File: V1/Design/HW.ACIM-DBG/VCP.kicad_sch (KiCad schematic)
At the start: 18 parts, among them J2 VCP ICSP, U3 PIC32MM0064GPM028

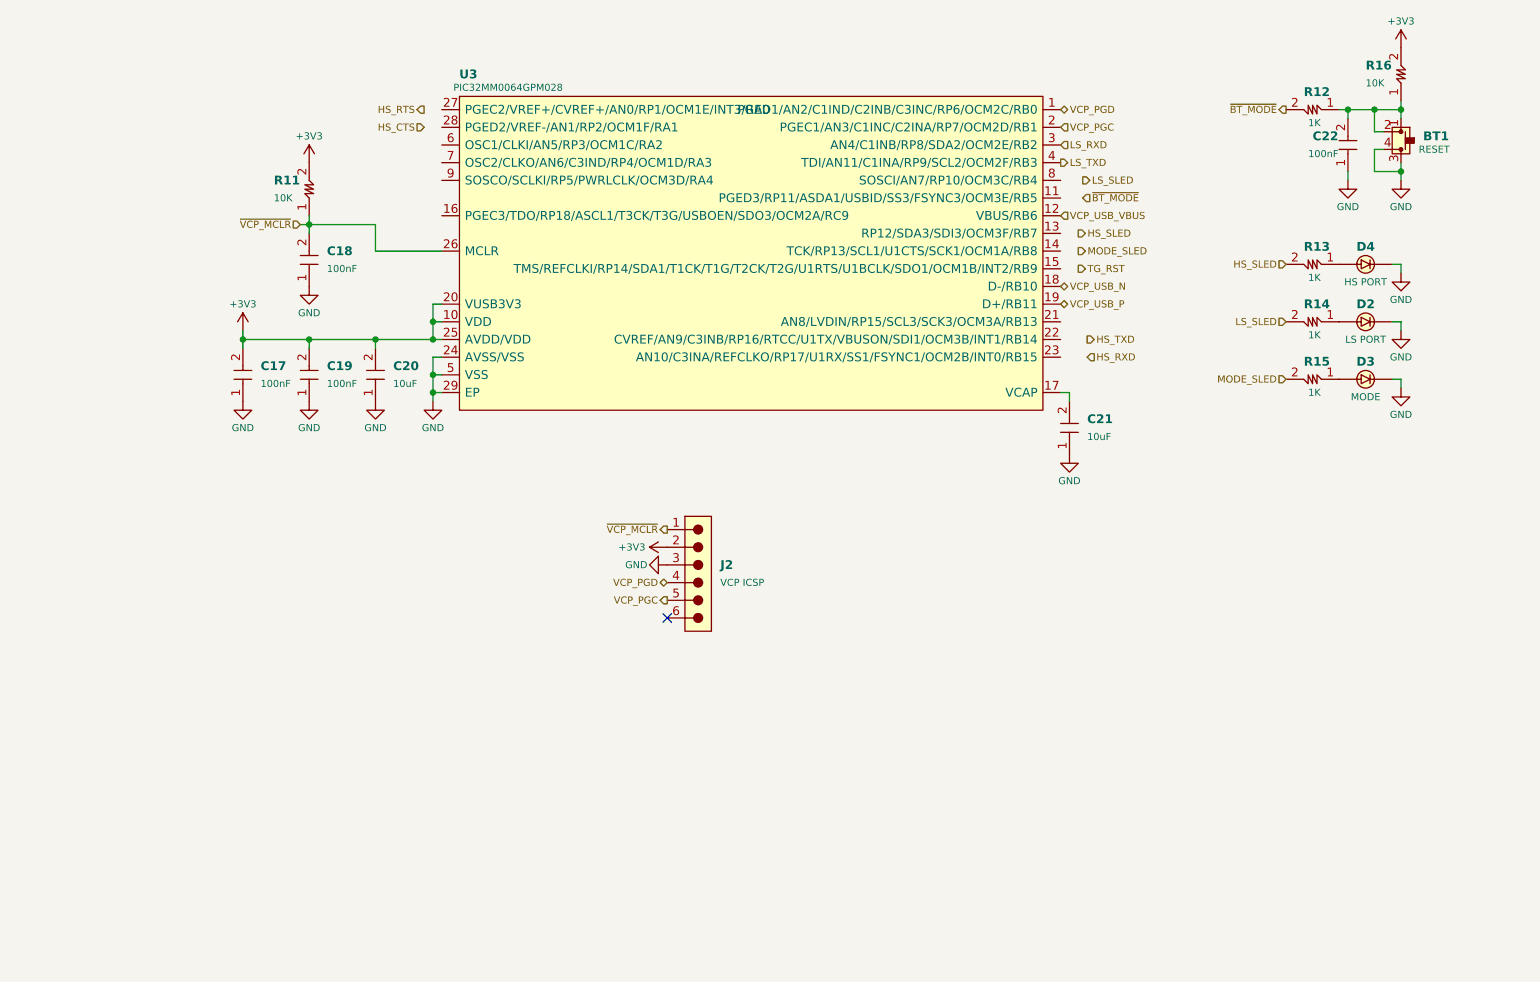
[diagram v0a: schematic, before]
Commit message: V1 layout update 2
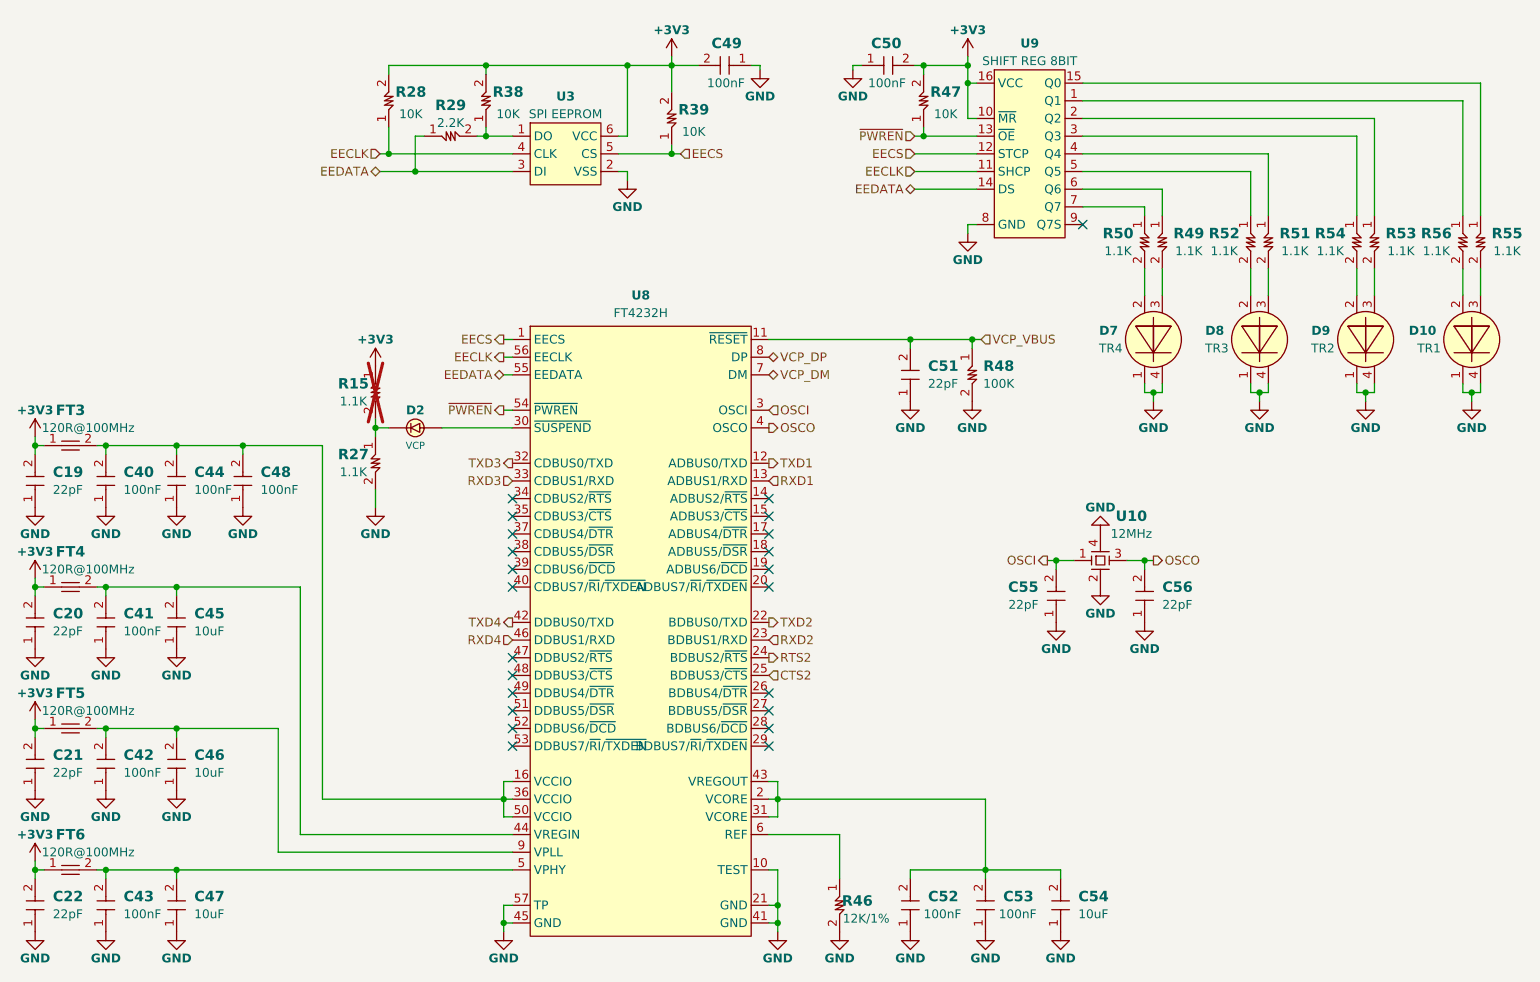
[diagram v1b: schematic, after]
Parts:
- removed BT1: RESET, SAMPI:BUTTON_4P_6x6, symbol SAMPI:BT
- removed C17, C18: 100nF, SAMPI:CAP0603, symbol SAMPI:CERCAP
- removed D3: MODE, SAMPI:LED3MM, symbol SAMPI:RLED
- removed D4: HS PORT, SAMPI:LED3MM, symbol SAMPI:YLED
- removed J2: VCP ICSP, SAMPI:HD-1x6x1.27MM-TH, symbol SAMPI:SIL06
- removed R11, R16: 10K, SAMPI:RES0603, symbol SAMPI:RES
- removed R12, R13, R14: 1K, SAMPI:RES0603, symbol SAMPI:RES
- removed U3: PIC32MM0064GPM028, SAMPI:UQFN28-4x4-EP, symbol TUANLIB:PIC32MM0256GPM028-I_M6
- added C40, C41, C42, C43, C44, C48, C49, C50, C52, C53: 100nF, SAMPI:CAP0603, symbol SAMPI:CERCAP
- added C45, C46, C47, C54: 10uF, SAMPI:CAP0603, symbol SAMPI:CERCAP
- added C51, C55, C56: 22pF, SAMPI:CAP0603, symbol SAMPI:CERCAP
- added D10: TR1, SAMPI:LED0606_4P, symbol SAMPI:RG_LED
- added D7: TR4, SAMPI:LED0606_4P, symbol SAMPI:RG_LED
- added D8: TR3, SAMPI:LED0606_4P, symbol SAMPI:RG_LED
- added D9: TR2, SAMPI:LED0606_4P, symbol SAMPI:RG_LED
- added FT3, FT4, FT5, FT6: 120R@100MHz, SAMPI:FT0603, symbol SAMPI:FerriteBead
- added R27, R49, R50, R51, R52, R53, R54, R55, R56: 1.1K, SAMPI:RES0603, symbol SAMPI:RES
- added R28, R38, R39, R47: 10K, SAMPI:RES0603, symbol SAMPI:RES
- added R29: 2.2K, SAMPI:RES0603, symbol SAMPI:RES
- added R46: 12K/1%, SAMPI:RES0603, symbol SAMPI:RES
- added R48: 100K, SAMPI:RES0603, symbol SAMPI:RES
- added U10: 12MHz, SAMPI:CDFN2520-ABM10, symbol SAMPI:XTAL-4P
- added U3: SPI EEPROM, SAMPI:SOT-23-6_MCHP, symbol SAMPI:93LC56
- added U8: FT4232H, SAMPI:VQFN-56_FTDI, symbol SAMPI:FT4232H
- added U9: SHIFT REG 8BIT, SAMPI:TSSOP16-SOT403-1, symbol SAMPI:74HC595
- C19, C22: value 100nF -> 22pF; MFT Samsung -> Walsin; MNP CL10B104KB8NNNC -> 0603N220J500CT
- C20, C21: value 10uF -> 22pF; MFT Samsung -> Walsin; MNP CL10A106MQ8NNNC -> 0603N220J500CT
- D2: value LS PORT -> VCP
- R15: value 1K -> 1.1K; MNP RC0603FR-071KL -> AC0603FR-071K1L; now not fitted; now left out of the parts list
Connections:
- net +3V3: now also C21.2, C22.2, R15.1, C49.2, C50.2, FT3.1, FT4.1, FT5.1, FT6.1, R28.2, R38.2, R39.2, R47.2, U3.6 (VCC), U9.10 (~{MR}), U9.16 (VCC)
- net GND: now also C40.1, C41.1, C42.1, C43.1, C44.1, C45.1, C46.1, C47.1, C48.1, C49.1, C50.1, C51.1, C52.1, C53.1, C54.1, C55.1, C56.1, D10.1 (GK), D10.4 (RK), D7.1 (GK), D7.4 (RK), D8.1 (GK), D8.4 (RK), D9.1 (GK), D9.4 (RK), R27.2, R46.2, R48.2, U10.2 (GND1), U10.4 (X2), U3.2 (VSS), U8.10 (TEST), U8.21 (GND), U8.41 (GND), U8.45 (GND), U8.57 (TP), U9.8 (GND); no longer D2.K
- net at D2.A: now also U8.30 (~{SUSPEND})
- net MODE_SLED: no longer names the net of R15.2
- net MODE_SLED: now also D2.K, R27.1
- new net: R49.1, U9.6 (Q6)
- new net: D7.3 (RA), R49.2
- new net: D10.2 (GA), R56.2
- new net: D10.3 (RA), R55.2
- new net: R53.1, U9.2 (Q2)
- new net: D9.3 (RA), R53.2
- new net: D7.2 (GA), R50.2
- new net: C52.2, C53.2, C54.2, U8.2 (VCORE), U8.31 (VCORE), U8.43 (VREGOUT)
- new net: C40.2, C44.2, C48.2, FT3.2, U8.16 (VCCIO), U8.36 (VCCIO), U8.50 (VCCIO)
- new net: C41.2, C45.2, FT4.2, U8.44 (VREGIN)
- new net: C43.2, C47.2, FT6.2, U8.5 (VPHY)
- new net: R46.1, U8.6 (REF)
- new net: C42.2, C46.2, FT5.2, U8.9 (VPLL)
- new net: R29.2, R38.1, U3.1 (DO)
- new net: D9.2 (GA), R54.2
- new net: R55.1, U9.15 (Q0)
- new net: R54.1, U9.3 (Q3)
- new net: R51.1, U9.4 (Q4)
- new net: D8.3 (RA), R51.2
- new net: R56.1, U9.1 (Q1)
- new net: R52.1, U9.5 (Q5)
- new net: R50.1, U9.7 (Q7)
- new net: D8.2 (GA), R52.2
- new net CTS2: U8.25 (BDBUS3/~{CTS})
- new net EECLK: R28.1, U3.4 (CLK), U8.56 (EECLK), U9.11 (SHCP)
- new net EECS: R39.1, U3.5 (CS), U8.1 (EECS), U9.12 (STCP)
- new net EEDATA: R29.1, U3.3 (DI), U8.55 (EEDATA), U9.14 (DS)
- new net OSCI: C55.2, U10.1 (X1), U8.3 (OSCI)
- new net OSCO: C56.2, U10.3 (GND2), U8.4 (OSCO)
- new net RTS2: U8.24 (BDBUS2/~{RTS})
- new net RXD1: U8.13 (ADBUS1/RXD)
- new net RXD2: U8.23 (BDBUS1/RXD)
- new net RXD3: U8.33 (CDBUS1/RXD)
- new net RXD4: U8.46 (DDBUS1/RXD)
- new net TXD1: U8.12 (ADBUS0/TXD)
- new net TXD2: U8.22 (BDBUS0/TXD)
- new net TXD3: U8.32 (CDBUS0/TXD)
- new net TXD4: U8.42 (DDBUS0/TXD)
- new net VCP_DM: U8.7 (DM)
- new net VCP_DP: U8.8 (DP)
- new net VCP_VBUS: C51.2, R48.1, U8.11 (~{RESET})
- new net ~{PWREN}: R47.1, U8.54 (~{PWREN}), U9.13 (~{OE})
- no-connect marks 1 -> 23
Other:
- moved on the sheet: D2
